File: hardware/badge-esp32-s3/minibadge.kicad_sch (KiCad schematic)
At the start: 2 parts

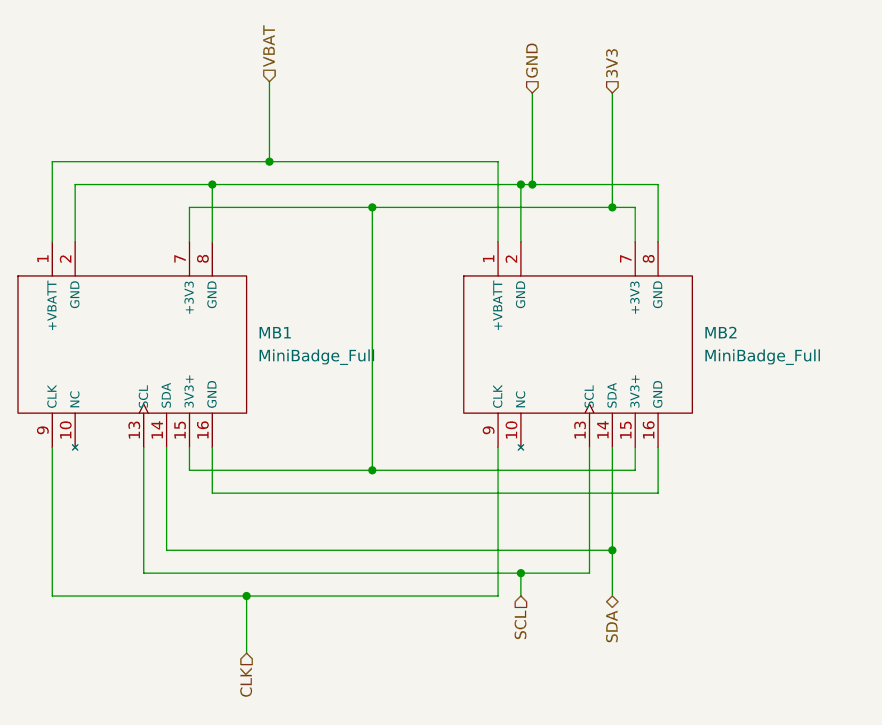
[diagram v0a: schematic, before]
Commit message: Finish schematic, start placing parts on layout
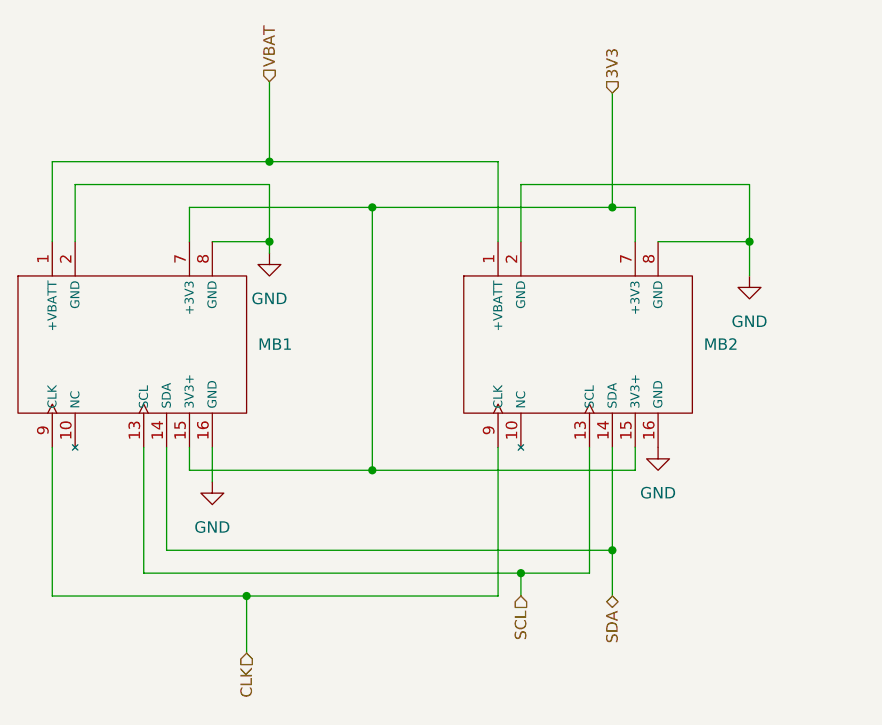
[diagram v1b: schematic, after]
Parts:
- removed MB1, MB2: MiniBadge_Full, symbol MiniBadge:MiniBadge_Full
- added MB1, MB2: MiniBadge_Full, minibadge:MiniBadge_Full_NoEdges, symbol minibadge:MiniBadge_Full
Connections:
- net 3V3: now also MB1.15 (3V3+), MB1.7 (+3V3), MB2.15 (3V3+), MB2.7 (+3V3)
- net CLK: now also MB1.9 (CLK), MB2.9 (CLK)
- net GND: now also MB1.16 (GND), MB1.2 (GND), MB1.8 (GND), MB2.16 (GND), MB2.2 (GND), MB2.8 (GND)
- net SCL: now also MB1.13 (SCL), MB2.13 (SCL)
- net SDA: now also MB1.14 (SDA), MB2.14 (SDA)
- net VBAT: now also MB1.1 (+VBATT), MB2.1 (+VBATT)
